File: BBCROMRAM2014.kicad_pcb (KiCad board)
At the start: 2 copper layers, 77.5 x 47 mm, 7 parts, among them J1 CON1, U1 74LS139, U2 29F010-DIL32, U3 W24512A, U4 27128, U5 74LS00, U6 27128

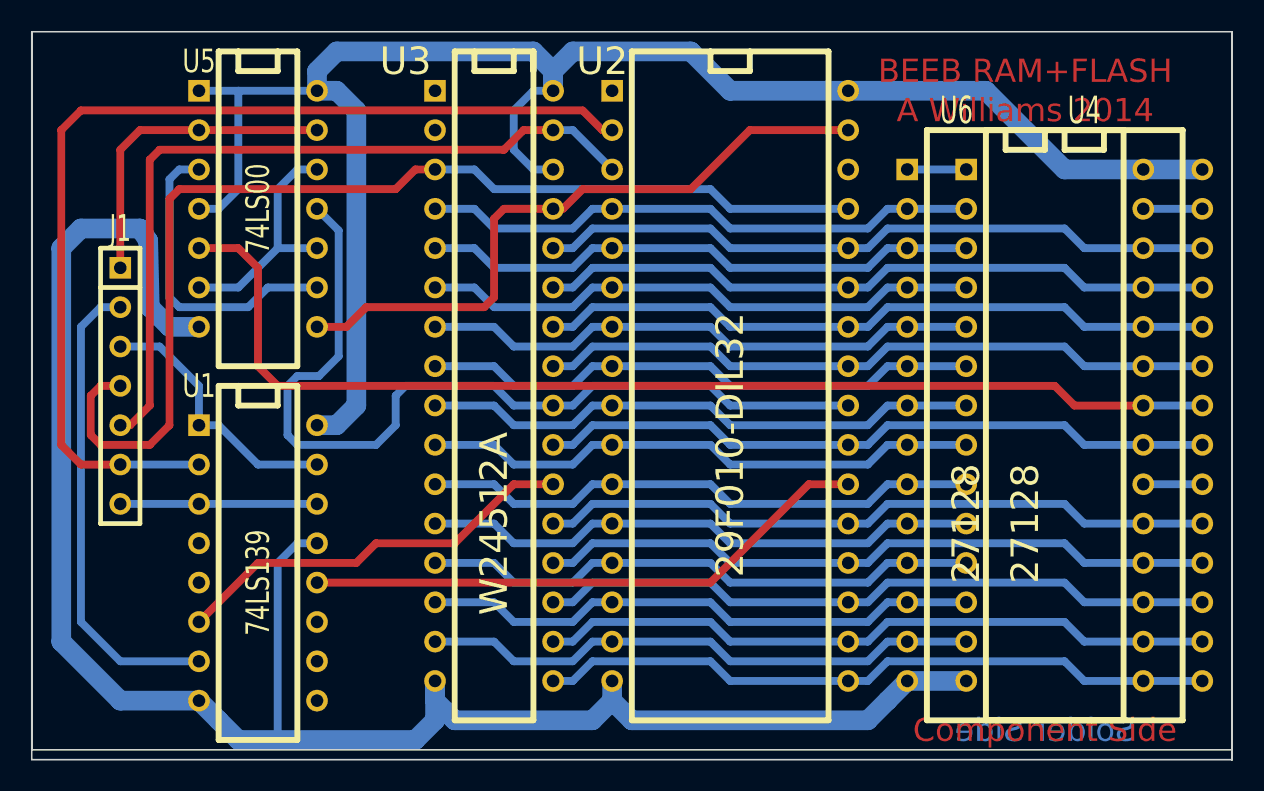
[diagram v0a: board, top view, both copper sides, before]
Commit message: First commit
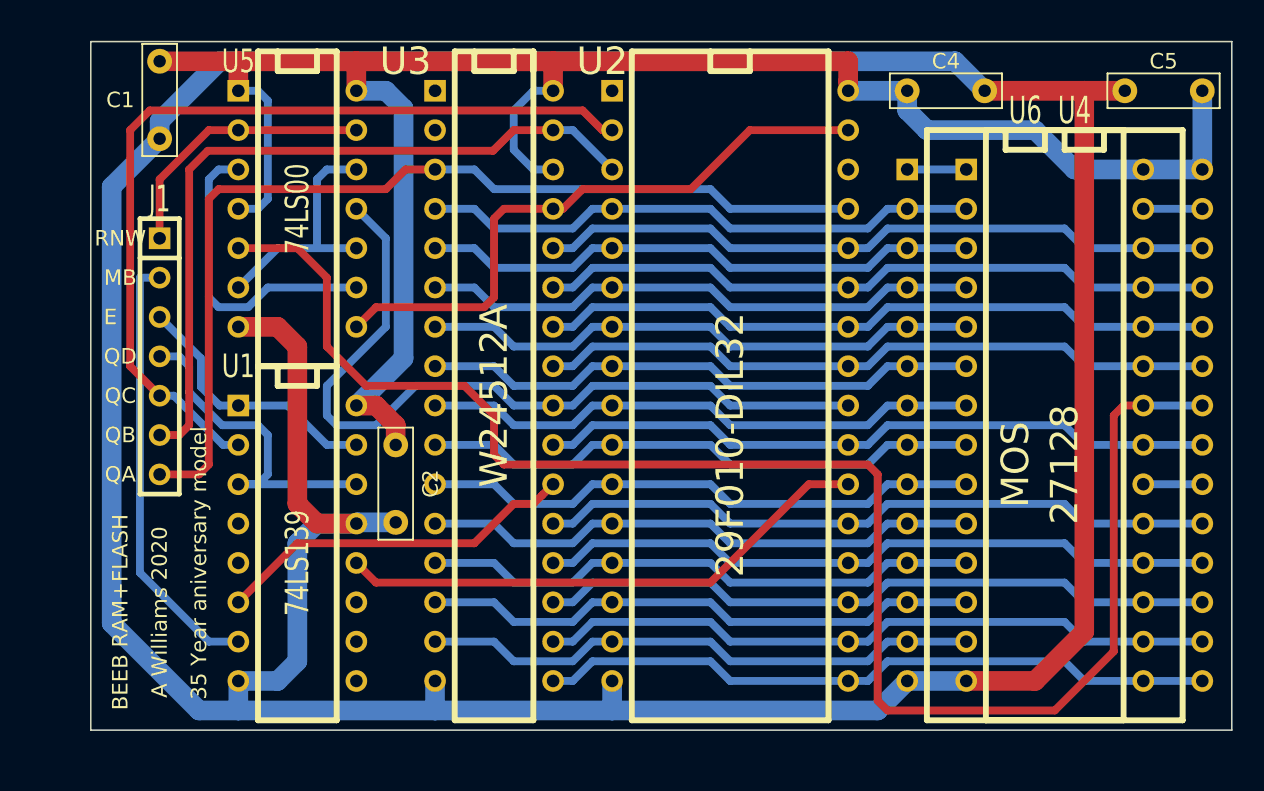
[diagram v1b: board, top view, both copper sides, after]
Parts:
- added C1: 0.1uF, Capacitor_THT:C_Rect_L7.0mm_W2.0mm_P5.00mm, F.Cu at (215.9, 98.4)
- added C2: 0.1uF, Capacitor_THT:C_Rect_L7.0mm_W2.0mm_P5.00mm, F.Cu at (231.1, 123.2)
- added C4: 0.1uF, Capacitor_THT:C_Rect_L7.0mm_W2.0mm_P5.00mm, F.Cu at (264.2, 100.3)
- added C5: 0.1uF, Capacitor_THT:C_Rect_L7.0mm_W2.0mm_P5.00mm, F.Cu at (283.2, 100.3)
- U4: value 27128 -> MOS
- moved J1 3.17 mm to (215.9, 117.5)
- moved U1 2.84 mm to (224.8, 129.5)
- moved U5 2.54 mm to (224.8, 108.0)
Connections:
- J1 pad 4: /QA -> /QD
- J1 pad 5: /QB -> /QC
- J1 pad 6: /QC -> /QB
- J1 pad 7: /QD -> /QA
- U1 pad 10: (no net) -> Net-(U1-Pad10)
- U1 pad 11: (no net) -> Net-(U1-Pad11)
- U1 pad 4: (no net) -> Net-(U1-Pad4)
- U1 pad 5: (no net) -> Net-(U1-Pad5)
- U1 pad 9: (no net) -> Net-(U1-Pad9)
- U3 pad 1: (no net) -> Net-(U3-Pad1)
- U3 pad 2: (no net) -> Net-(U3-Pad2)
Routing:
- net GND: track 123.7 -> 244.0 mm
- net /MOE: track 72.7 -> 104.3 mm
- net VCC: track 116.6 -> 130.5 mm
- net /QC: track 66.3 -> 56.5 mm
- net /QD: track 12.7 -> 22.4 mm
- net /QA: track 70.8 -> 63.7 mm
- net /NOE: track 58.1 -> 52.3 mm
- net /NRAMCS: track 26.5 -> 23.5 mm
- net /RNW: track 20.8 -> 17.8 mm
- net /NWDS: track 42.5 -> 40.0 mm
- net /MB: track 30.8 -> 28.5 mm
- net /NFLASHCS: track 36.9 -> 34.9 mm
- net /QB: track 50.0 -> 48.1 mm
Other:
- board size 77.5 x 47 mm -> 73.7 x 44.4 mm
- board text added: "35 Year aniversary model"
- board text added: "A Williams 2020"
- board text added: "E"
- board text added: "MB"
- board text added: "QA"
- board text added: "QB"
- board text added: "QC"
- board text added: "QD"
- board text added: "RNW"
- board text removed: "A Williams 2014"
- board text removed: "Component Side"
- board text removed: "Solder Side"
